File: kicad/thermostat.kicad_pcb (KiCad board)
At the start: 2 copper layers, 108 x 80 mm, 19 parts, among them J1 Display i2c, J2 Sensor i2c, J3 PoE Input, J4 PoE Output, J5 0857891001

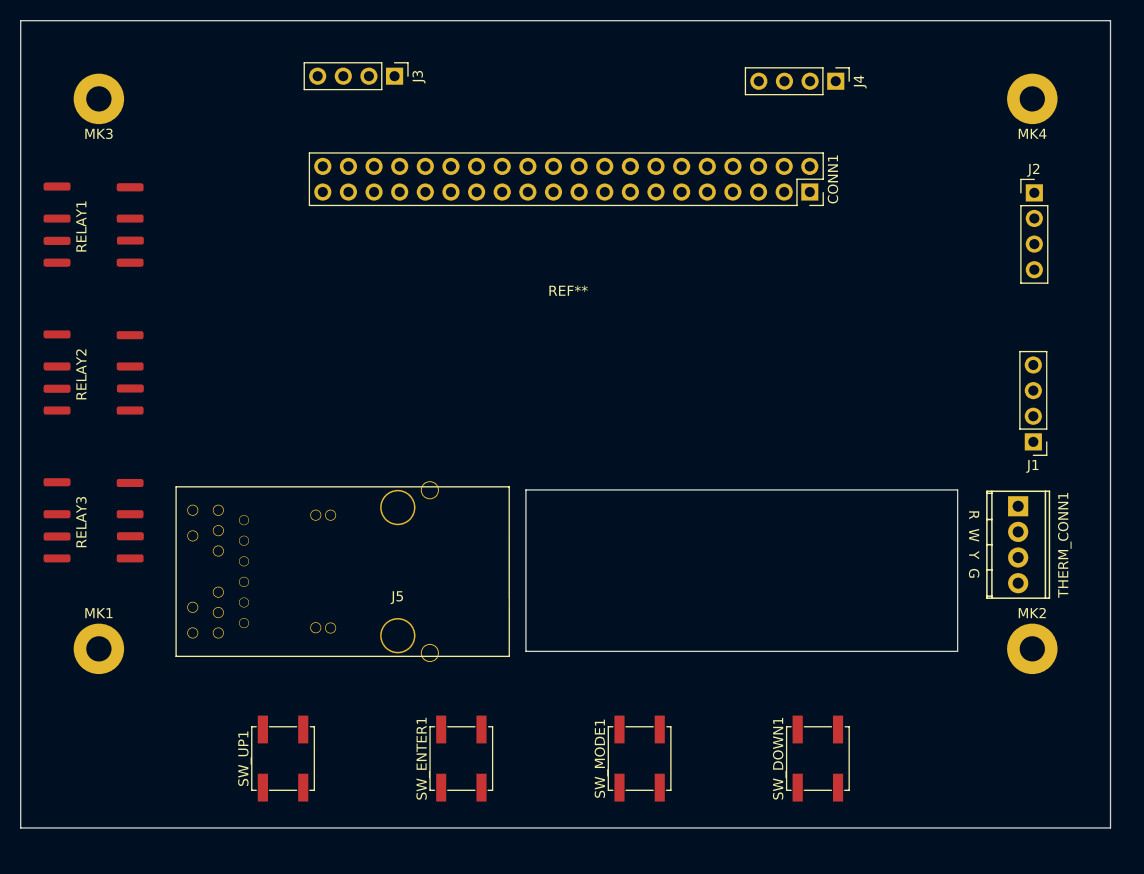
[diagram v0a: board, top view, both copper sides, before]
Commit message: more updates, backstop before 24v conversation
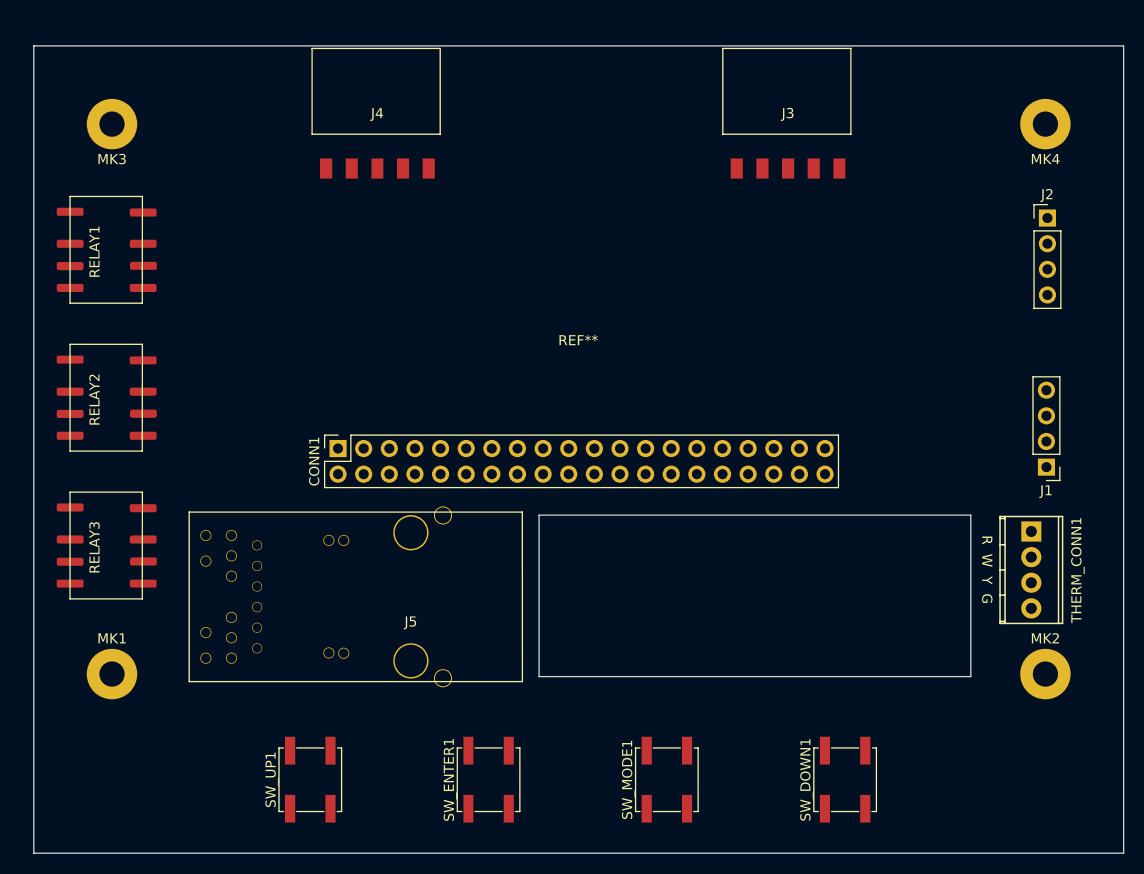
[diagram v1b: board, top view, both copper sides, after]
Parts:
- J3, J4: footprint Pin_Headers:Pin_Header_Straight_1x04_Pitch2.54mm -> project_footprints:M20-7910542R
- moved CONN1 53.2 mm to (176.0, 150.3), turned to 90 degrees
- moved J4 45.5 mm to (179.9, 116.6), turned to 0 degrees
- moved J3 39.1 mm to (220.6, 116.6), turned to 0 degrees
- moved REF** 5.00 mm to (199.8, 140.1)
- moved SW_MODE1 3.42 mm to (208.6, 183.1)
- moved SW_DOWN1 3.42 mm to (226.2, 183.1)
- moved SW_ENTER1 3.42 mm to (190.9, 183.1)
- moved SW_UP1 3.42 mm to (173.2, 183.1)
- moved J2 2.82 mm to (246.3, 127.5)
- moved J5 2.82 mm to (183.2, 165.0)
- moved RELAY1 2.82 mm to (152.4, 130.8)
- moved RELAY2 2.82 mm to (152.4, 145.4)
- moved RELAY3 2.82 mm to (152.4, 160.1)
- moved J1 2.82 mm to (246.2, 152.1)
- moved MK1 2.82 mm to (153.6, 172.7)
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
